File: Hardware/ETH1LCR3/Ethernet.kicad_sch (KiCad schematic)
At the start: 36 parts, among them U201 LAN8742A, U202 SRV05-4, Y201 NX5032GA-25

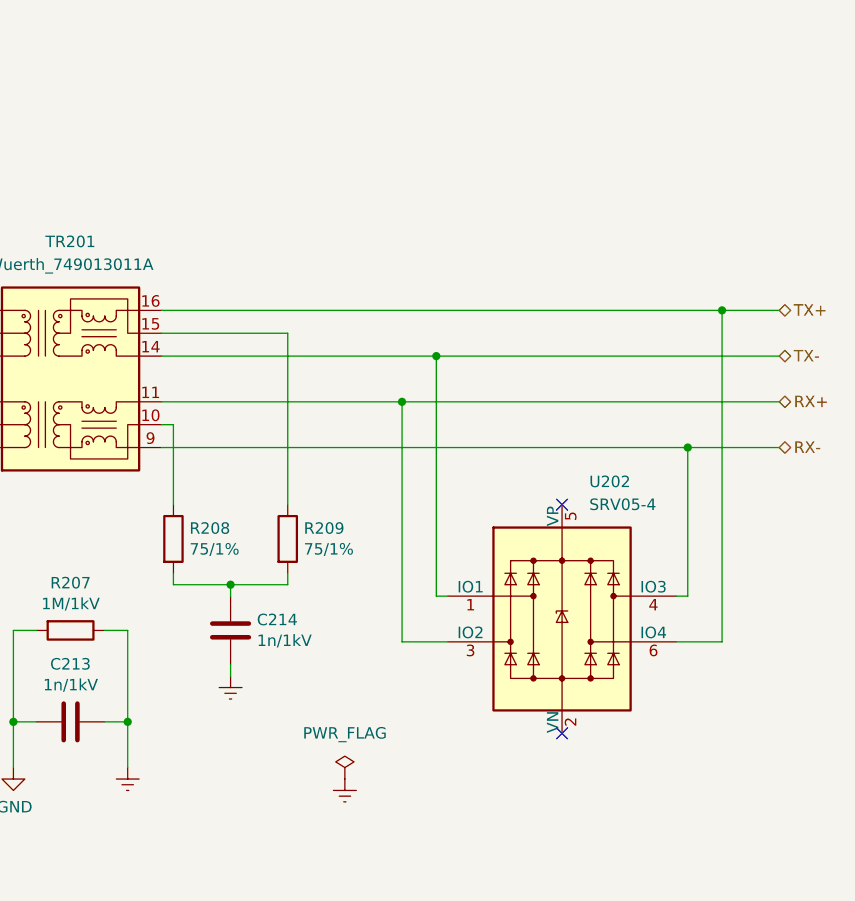
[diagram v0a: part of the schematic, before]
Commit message: PCB layout
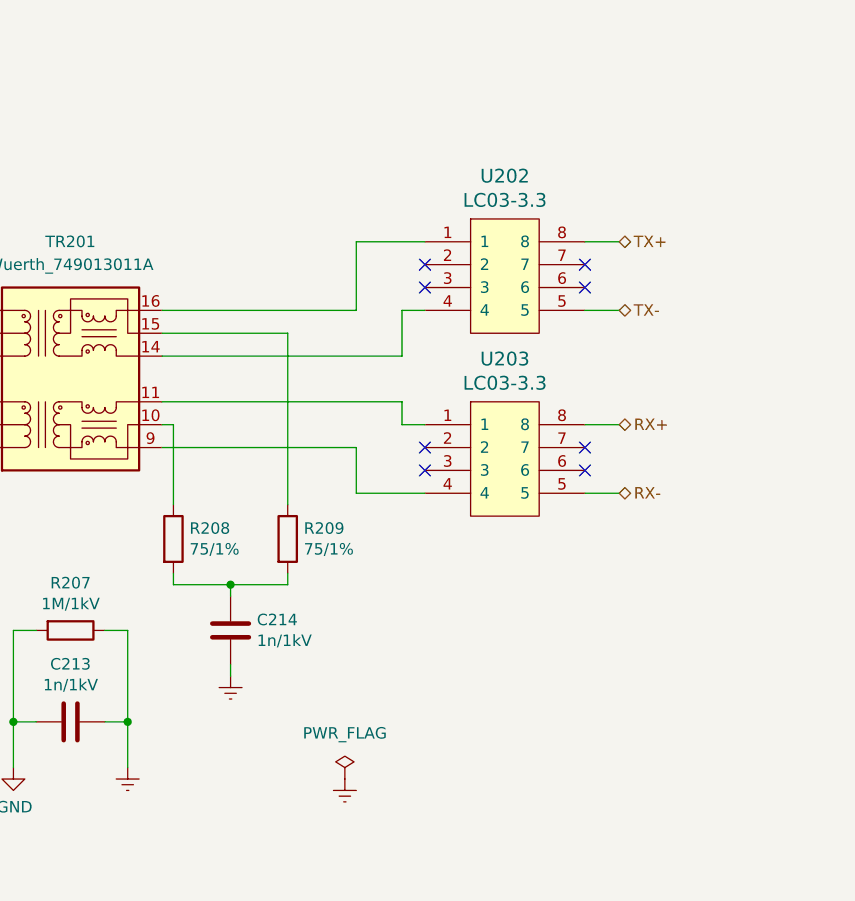
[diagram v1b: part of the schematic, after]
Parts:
- removed U202: SRV05-4, Package_TO_SOT_SMD:SOT-23-6, symbol Power_Protection:SRV05-4
- added U202, U203: LC03-3.3, Package_SO:SOIC-8_3.9x4.9mm_P1.27mm, symbol ETH1CSMU2:LC03-3.3
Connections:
- net RX+: now also U203.8; no longer TR201.11 (RX+)
- net RX-: now also U203.5; no longer TR201.9 (RX-)
- net TX+: now also U202.8; no longer TR201.16 (TX+)
- net TX-: now also U202.5; no longer TR201.14 (TX-)
- new net: TR201.16 (TX+), U202.1
- new net: TR201.14 (TX-), U202.4
- new net: TR201.11 (RX+), U203.1
- new net: TR201.9 (RX-), U203.4
- no-connect marks 2 -> 8

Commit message: Updated project to KiCAD 9
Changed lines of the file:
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@@
 (kicad_sch
-	(version 20231120)
+	(version 20250114)
 	(generator "eeschema")
-	(generator_version "8.0")
+	(generator_version "9.0")
 	(paper "A4")
 	(junction
@@
 	(label "ETH_TXP"
 		(at 107.95 71.12 180)
-		(fields_autoplaced yes)
 		(effects
 			(font
@@
 	(label "MODE1"
 		(at 60.96 179.07 90)
-		(fields_autoplaced yes)
 		(effects
 			(font
@@
 	(label "RMII_MDIO"
 		(at 48.26 86.36 0)
-		(fields_autoplaced yes)
 		(effects
 			(font
@@
 	(label "MODE0"
 		(at 58.42 179.07 90)
-		(fields_autoplaced yes)
 		(effects
 			(font
@@
 	(label "ETH_RXP"
 		(at 107.95 76.2 180)
-		(fields_autoplaced yes)
 		(effects
 			(font
@@
 	(label "ETH_RXN"
 		(at 107.95 78.74 180)
-		(fields_autoplaced yes)
 		(effects
 			(font
@@
 	(label "LED1"
 		(at 102.87 91.44 180)
-		(fields_autoplaced yes)
 		(effects
 			(font
@@
 	(label "MODE1"
 		(at 52.07 78.74 0)
-		(fields_autoplaced yes)
 		(effects
 			(font
@@
 	(label "MODE2"
 		(at 52.07 83.82 0)
-		(fields_autoplaced yes)
 		(effects
 			(font
@@
 	(label "MODE0"
 		(at 52.07 76.2 0)
-		(fields_autoplaced yes)
 		(effects
 			(font
@@
 	(label "RMII_MDIO"
 		(at 86.36 177.8 90)
-		(fields_autoplaced yes)
 		(effects
 			(font
@@
 	(label "LED2"
 		(at 102.87 93.98 180)
-		(fields_autoplaced yes)
 		(effects
 			(font
@@
 	(label "REFCLK0"
 		(at 49.53 96.52 0)
-		(fields_autoplaced yes)
 		(effects
 			(font
@@
 	(label "REFCLK0"
 		(at 66.04 179.07 90)
-		(fields_autoplaced yes)
 		(effects
 			(font
@@
 	(label "MODE2"
 		(at 63.5 179.07 90)
-		(fields_autoplaced yes)
 		(effects
 			(font
@@
 	(label "ETH_TXN"
 		(at 107.95 73.66 180)
-		(fields_autoplaced yes)
 		(effects
 			(font
@@
 		(shape bidirectional)
 		(at 257.81 71.12 0)
-		(fields_autoplaced yes)
 		(effects
 			(font
@@
 		(shape bidirectional)
 		(at 27.94 71.12 180)
-		(fields_autoplaced yes)
 		(effects
 			(font
@@
 		(shape bidirectional)
 		(at 27.94 83.82 180)
-		(fields_autoplaced yes)
 		(effects
 			(font
@@
 		(shape bidirectional)
 		(at 257.81 63.5 0)
-		(fields_autoplaced yes)
 		(effects
 			(font
@@
 		(shape bidirectional)
 		(at 27.94 88.9 180)
-		(fields_autoplaced yes)
 		(effects
 			(font
@@
 		(shape bidirectional)
 		(at 27.94 81.28 180)
-		(fields_autoplaced yes)
 		(effects
 			(font
@@
 		(shape bidirectional)
 		(at 27.94 78.74 180)
-		(fields_autoplaced yes)
 		(effects
 			(font
@@
 		(shape bidirectional)
 		(at 257.81 91.44 0)
-		(fields_autoplaced yes)
 		(effects
 			(font
@@
 		(shape bidirectional)
 		(at 27.94 91.44 180)
-		(fields_autoplaced yes)
 		(effects
 			(font
@@
 		(shape bidirectional)
 		(at 27.94 68.58 180)
-		(fields_autoplaced yes)
 		(effects
 			(font
@@
 		(shape bidirectional)
 		(at 27.94 73.66 180)
-		(fields_autoplaced yes)
 		(effects
 			(font
@@
 		(shape bidirectional)
 		(at 27.94 93.98 180)
-		(fields_autoplaced yes)
 		(effects
 			(font
@@
 		(shape bidirectional)
 		(at 257.81 83.82 0)
-		(fields_autoplaced yes)
 		(effects
 			(font
@@
 		(shape bidirectional)
 		(at 27.94 76.2 180)
-		(fields_autoplaced yes)
-		(effects
-			(font
+		(effects
+			(font
